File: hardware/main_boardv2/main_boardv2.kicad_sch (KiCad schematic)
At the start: 4 parts

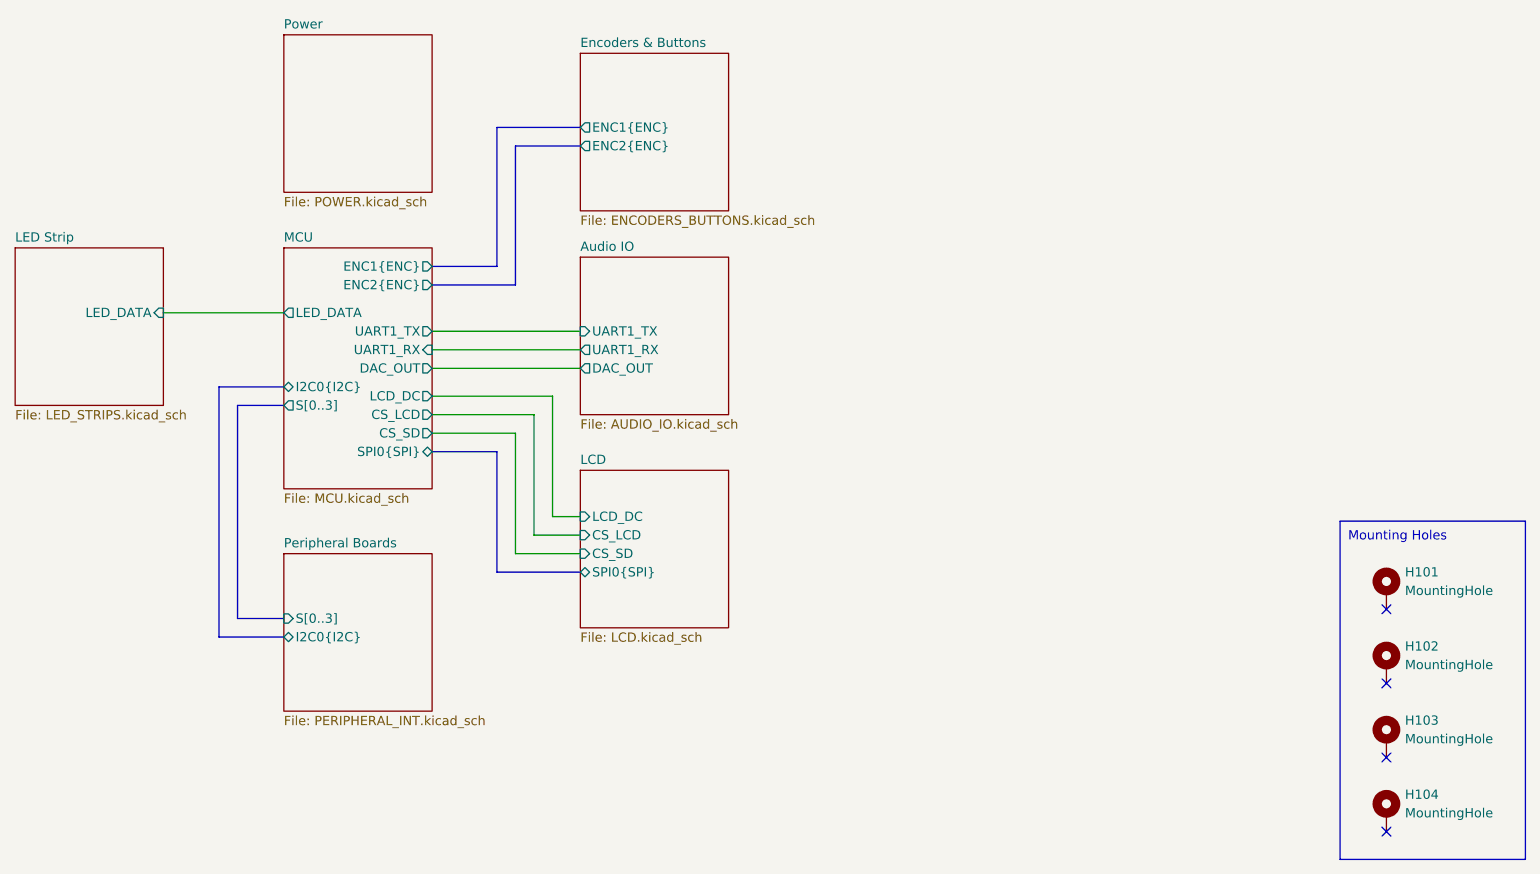
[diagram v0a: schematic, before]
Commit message: new hardware
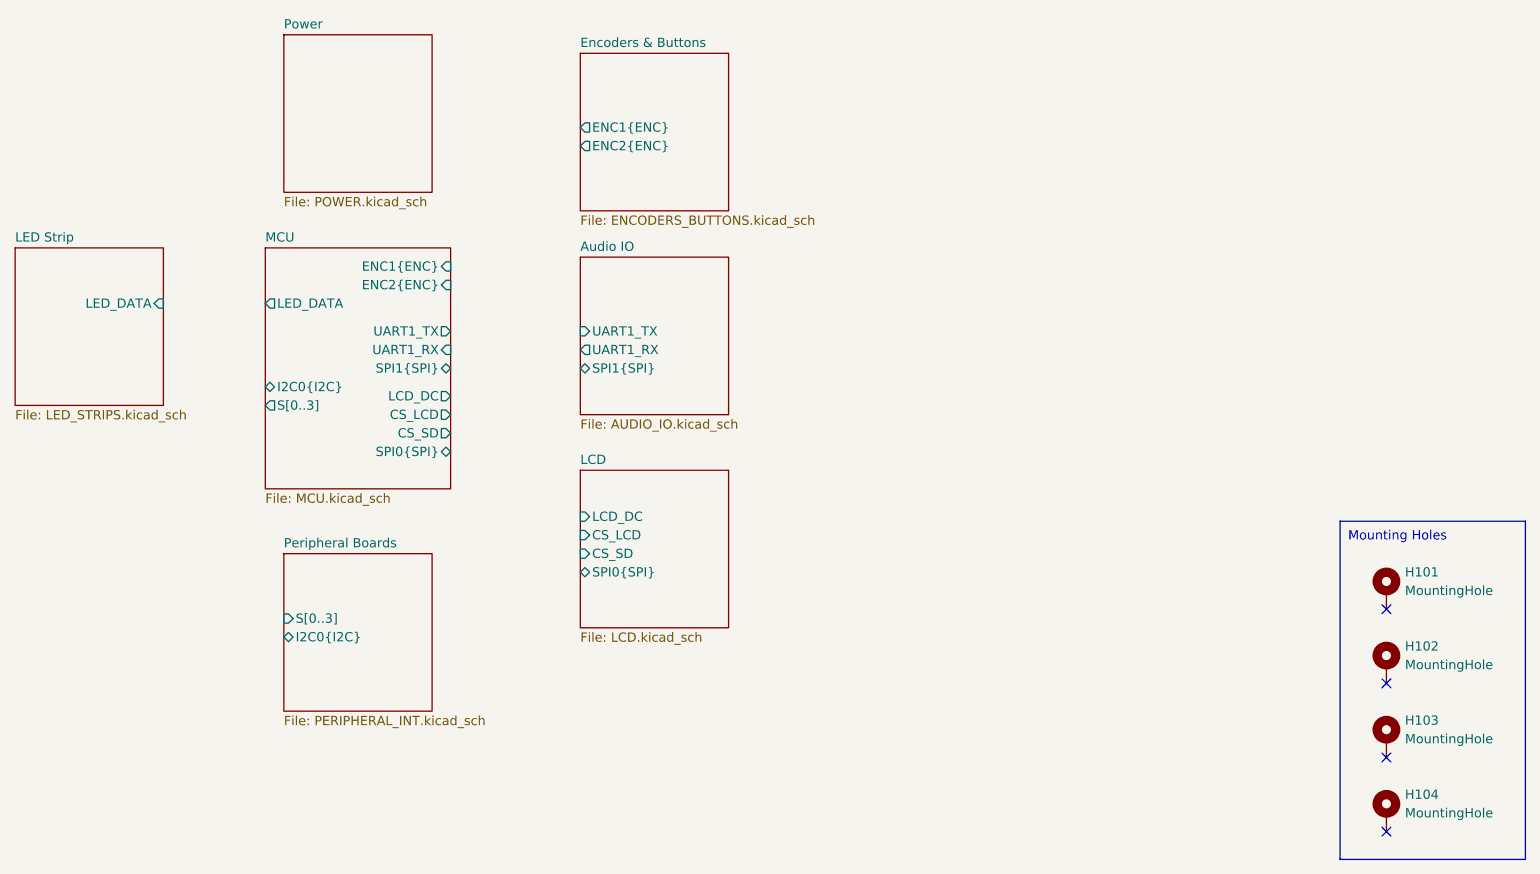
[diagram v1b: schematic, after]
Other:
- sheet Audio IO ports: added SPI1{SPI}; removed DAC_OUT
- sheet MCU ports: added SPI1{SPI}; removed DAC_OUT
